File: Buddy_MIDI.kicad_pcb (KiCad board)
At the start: 2 copper layers, 41.4 x 32 mm, 22 parts, among them J1 AudioJack3, J2 AudioJack3, J3 Conn_01x04_Socket, Q2 2N2222, U1 4N25, U2 SN74LVC1G14DBV

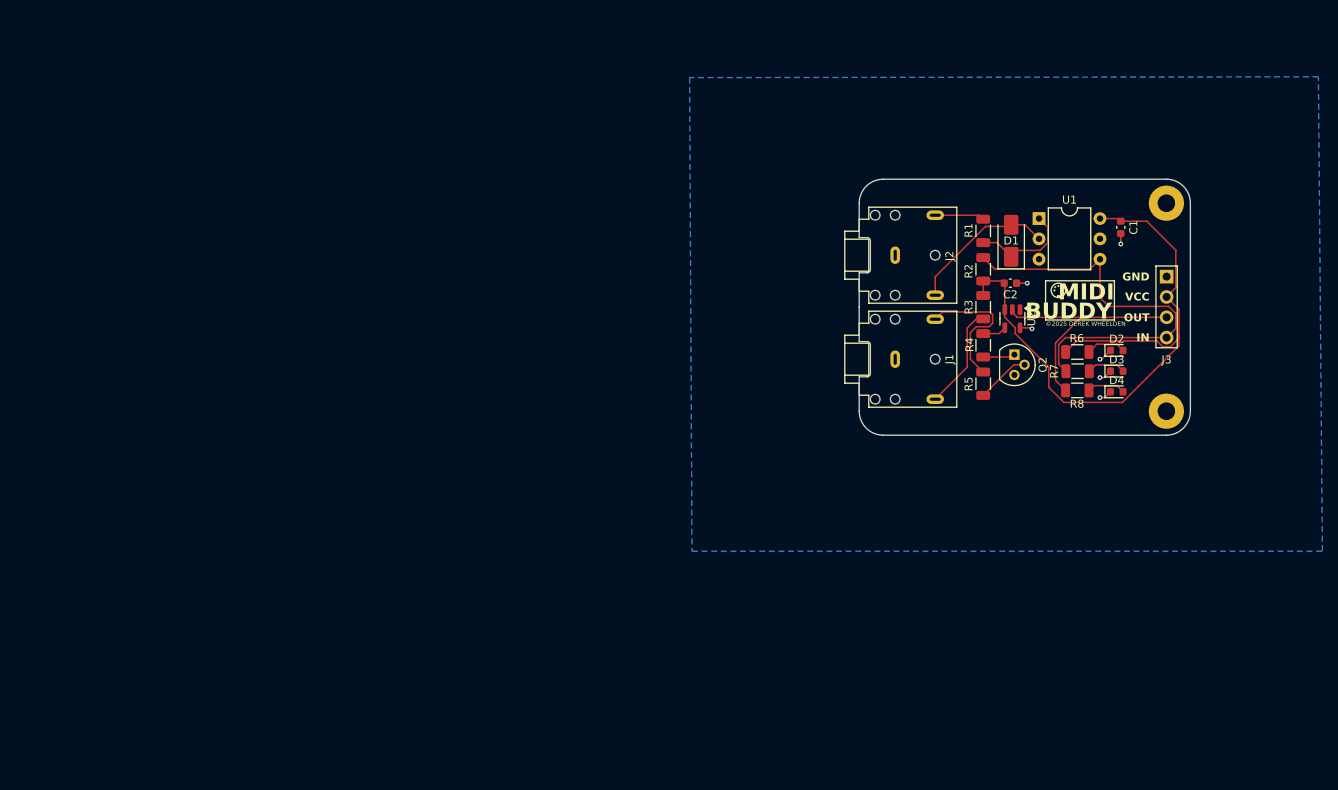
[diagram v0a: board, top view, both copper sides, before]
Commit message: New form factor
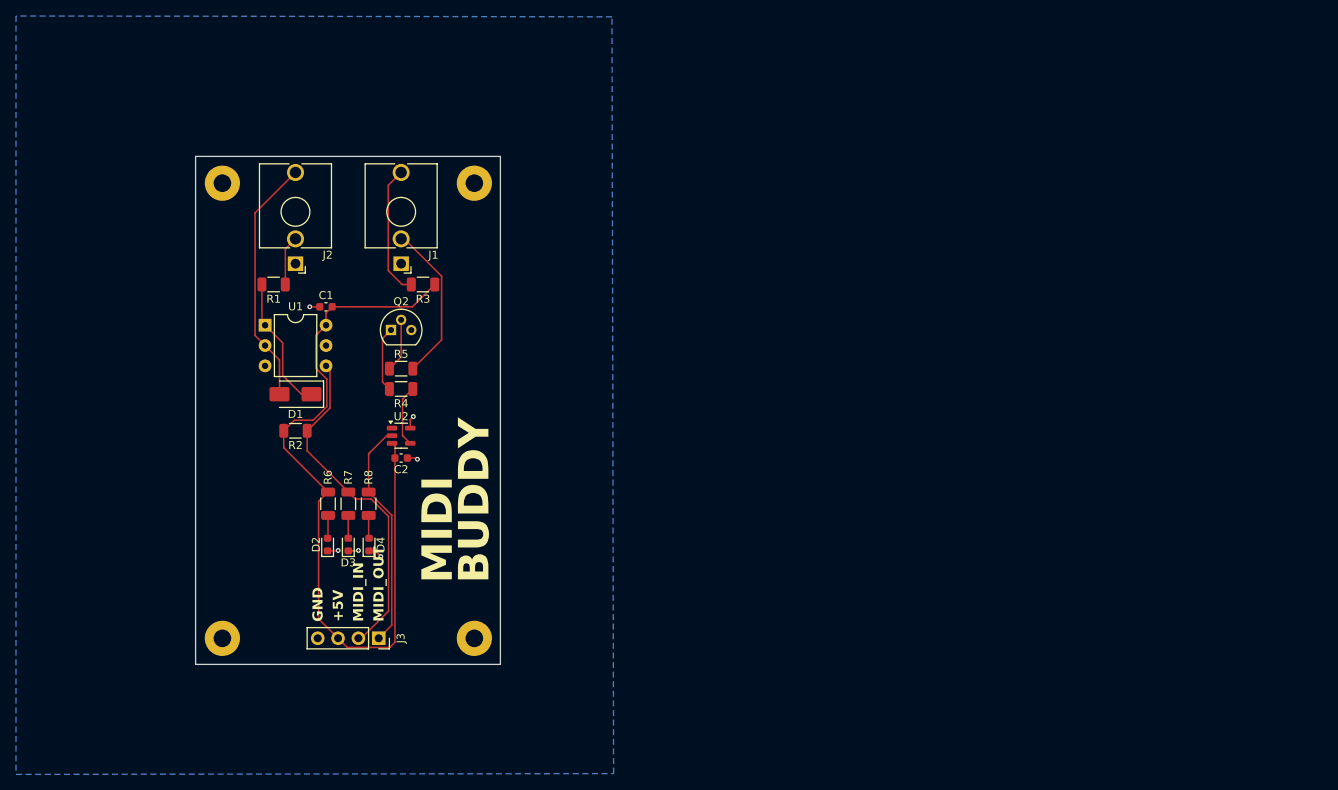
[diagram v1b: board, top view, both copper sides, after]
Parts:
- removed REF** (x2): MountingHole_2.2mm_M2_Pad, MountingHole:MountingHole_2.2mm_M2_Pad
- added H1: MountingHole_Pad, MountingHole:MountingHole_2.2mm_M2_Pad, F.Cu at (88.4, 86.4)
- added H2: MountingHole_Pad, MountingHole:MountingHole_2.2mm_M2_Pad, F.Cu at (119.9, 86.4)
- added H3: MountingHole_Pad, MountingHole:MountingHole_2.2mm_M2_Pad, F.Cu at (88.4, 143.3)
- added H4: MountingHole_Pad, MountingHole:MountingHole_2.2mm_M2_Pad, F.Cu at (119.9, 143.3)
- J1, J2: footprint Connector_Audio:Jack_3.5mm_CUI_SJ1-3523N_Horizontal -> Connector_Audio:Jack_3.5mm_QingPu_WQP-PJ398SM_Vertical_CircularHoles
- moved J3 105.4 mm to (107.9, 143.3), turned to -90 degrees
- moved D2 101.6 mm to (101.5, 131.6), turned to 90 degrees
- moved C1 99.8 mm to (101.3, 101.9), turned to 0 degrees
- moved D3 98.5 mm to (104.1, 131.6), turned to 90 degrees
- moved U1 97.7 mm to (93.7, 104.2)
- moved R6 95.6 mm to (101.6, 126.5), turned to -90 degrees
- moved D4 95.4 mm to (106.7, 131.6), turned to 90 degrees
- moved R7 92.7 mm to (104.1, 126.5), turned to -90 degrees
- moved D1 91.5 mm to (97.5, 112.8), turned to 180 degrees
- moved R8 89.7 mm to (106.7, 126.5), turned to -90 degrees
- moved R1 88.9 mm to (94.8, 99.1), turned to 180 degrees
- moved R2 88.3 mm to (97.5, 117.3), turned to 180 degrees
- moved C2 79.2 mm to (110.7, 120.8)
- moved Q2 78.0 mm to (109.5, 104.8), turned to 0 degrees
- moved U2 77.8 mm to (110.7, 118.0), turned to 0 degrees
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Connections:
- J3 pad 1: MIDI_IN -> MIDI_OUT
- J3 pad 2: MIDI_OUT -> MIDI_IN
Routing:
- net VCC: track 79.9 -> 97.1 mm
- net Net-(D1-A): track 18.7 -> 31.1 mm
- net MIDI_IN: track 51.9 -> 42.6 mm
- net Net-(R4-Pad1): track 3.00 -> 7.72 mm
- net Net-(Q2-B): track 4.02 -> 8.16 mm
- net Net-(D1-K): track 13.0 -> 17.0 mm
- net Net-(J1-PadT): track 13.0 -> 16.5 mm
- net Net-(J1-PadR): track 17.6 -> 20.0 mm
- net Net-(D2-A): track 4.99 -> 2.88 mm
- net MIDI_OUT: track 31.1 -> 29.0 mm
- net Net-(D3-A): track 4.87 -> 2.86 mm
- net Net-(D4-A): track 4.83 -> 2.88 mm
- net GND: track 9.20 -> 8.58 mm
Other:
- board size 41.4 x 32 mm -> 38.1 x 63.5 mm
- board text added: "+5V"
- board text added: "MIDI_IN"
- board text added: "MIDI_OUT"
- board text removed: "IN"
- board text removed: "OUT"
- board text removed: "VCC"
- board text removed: "©2025 DEREK WHEELDEN"
